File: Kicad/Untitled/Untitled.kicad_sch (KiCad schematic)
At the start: 10 parts, among them J1 Conn_01x16_Pin, P1 USB_C_Plug_USB2.0, U1 NCP1117-3.3_TO252, U2 ESP32-S3, Y1 ABM8-40.000MHZ-B2-T

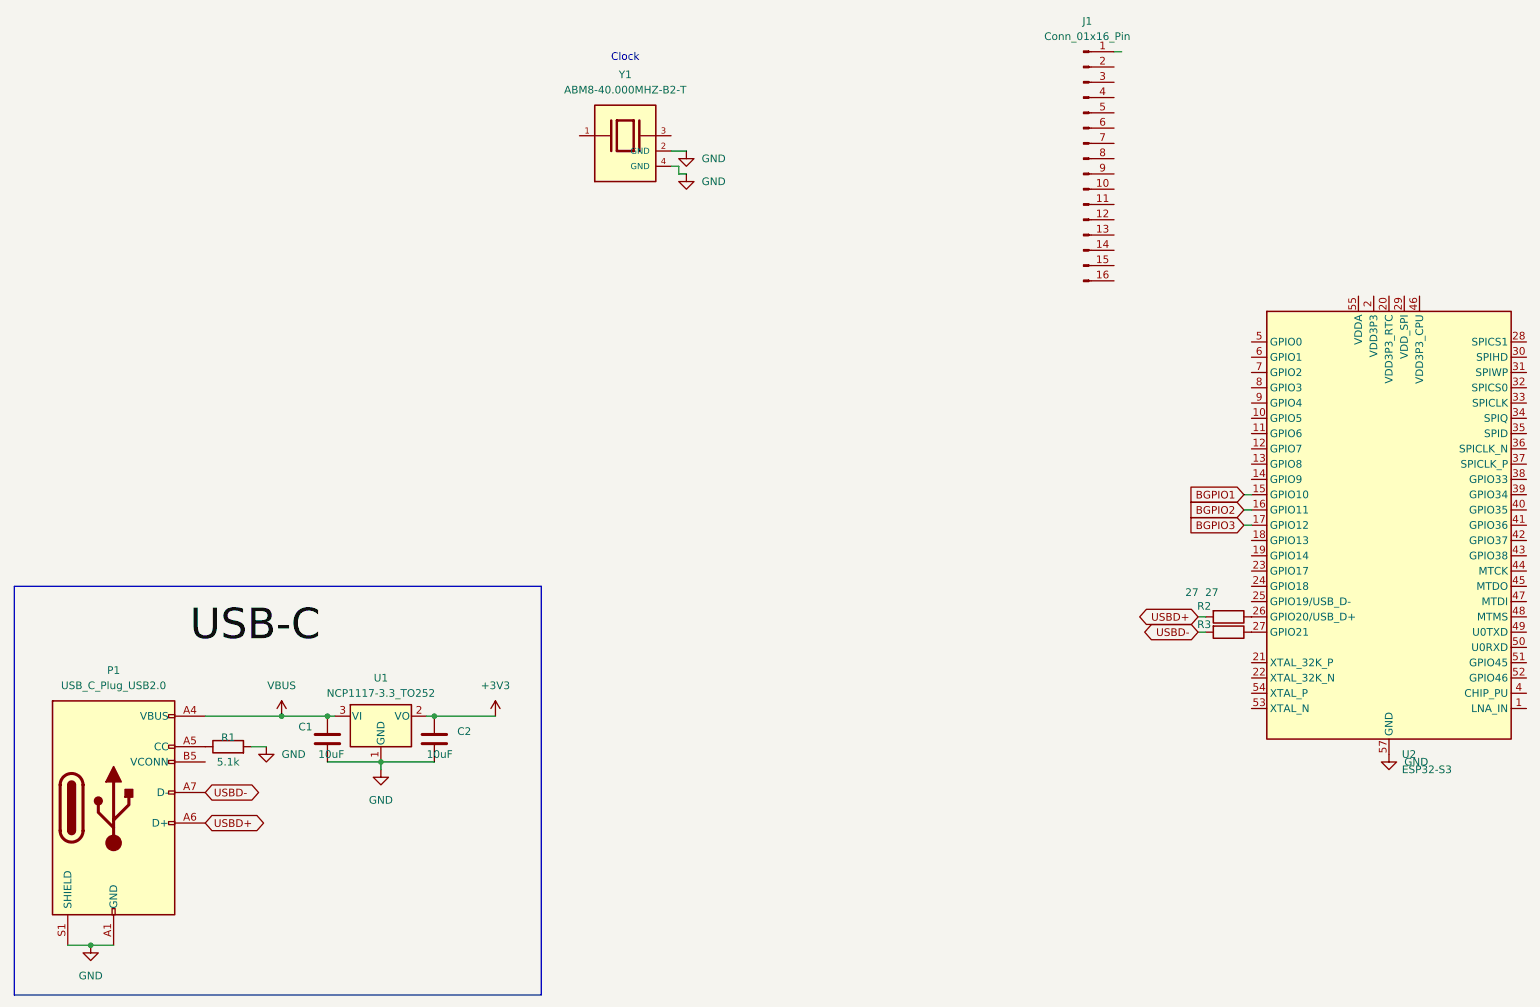
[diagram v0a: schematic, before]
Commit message: update schematic, more info in journakl
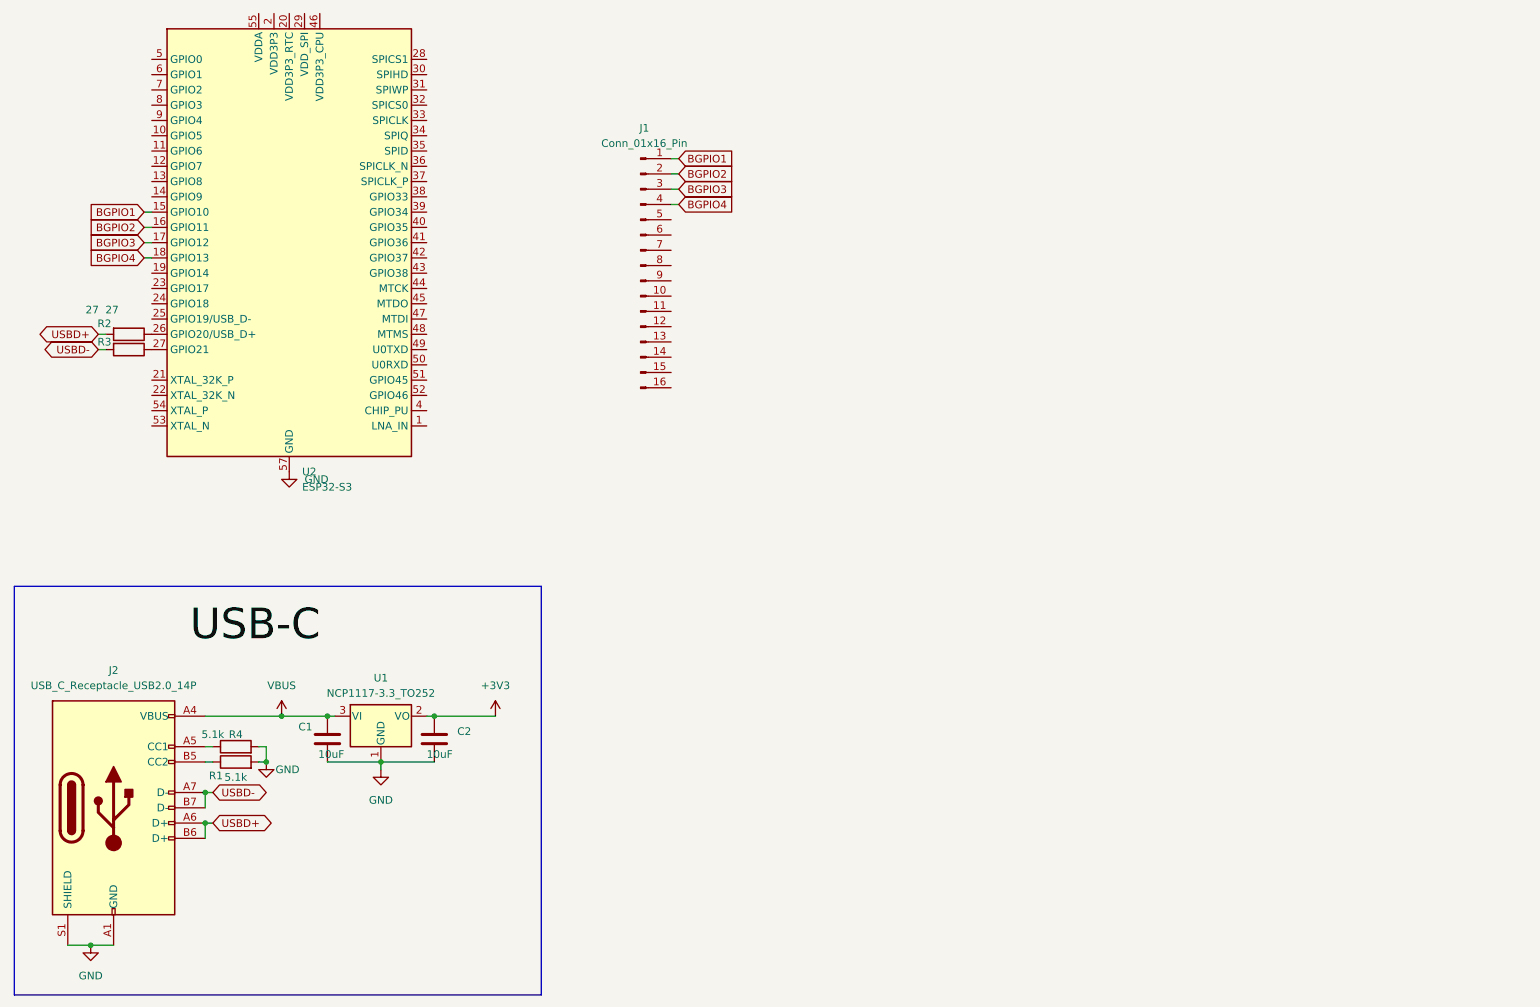
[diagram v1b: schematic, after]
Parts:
- removed P1: USB_C_Plug_USB2.0, symbol Connector:USB_C_Plug_USB2.0
- removed Y1: ABM8-40.000MHZ-B2-T, ABM8-40.000MHZ-B2-T:XTAL_ABM8-40.000MHZ-B2-T, symbol ABM8-40.000MHZ-B2-T:ABM8-40.000MHZ-B2-T
- added J2: USB_C_Receptacle_USB2.0_14P, symbol Connector:USB_C_Receptacle_USB2.0_14P
- added R4: 5.1k, symbol Device:R
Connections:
- net BGPIO1: now also J1.1 (Pin_1)
- net BGPIO2: now also J1.2 (Pin_2)
- net BGPIO3: now also J1.3 (Pin_3)
- net GND: now also J2.A1 (GND), J2.A12 (GND), J2.B1 (GND), J2.B12 (GND), J2.S1 (SHIELD), R4.2
- net USBD+: now also J2.A6 (D+), J2.B6 (D+)
- net USBD-: now also J2.A7 (D-), J2.B7 (D-)
- net VBUS: now also J2.A4 (VBUS), J2.A9 (VBUS), J2.B4 (VBUS), J2.B9 (VBUS)
- net at R1.1: now also J2.B5 (CC2)
- net BGPIO4: now reaches J1.4 (Pin_4)
- net BGPIO4: now also U2.18 (GPIO13)
- new net: J2.A5 (CC1), R4.1
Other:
- note removed: "Clock"
- moved on the sheet: J1, R1, R2, R3, U2
